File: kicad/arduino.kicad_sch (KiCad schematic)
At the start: 23 parts, among them J1 USB_B, J2 Conn_02x03_Odd_Even, SW1 Reset, U5 ATmega328P-A, U6 CH340C, U7 AMS1117-5.0, Y1 16MHz

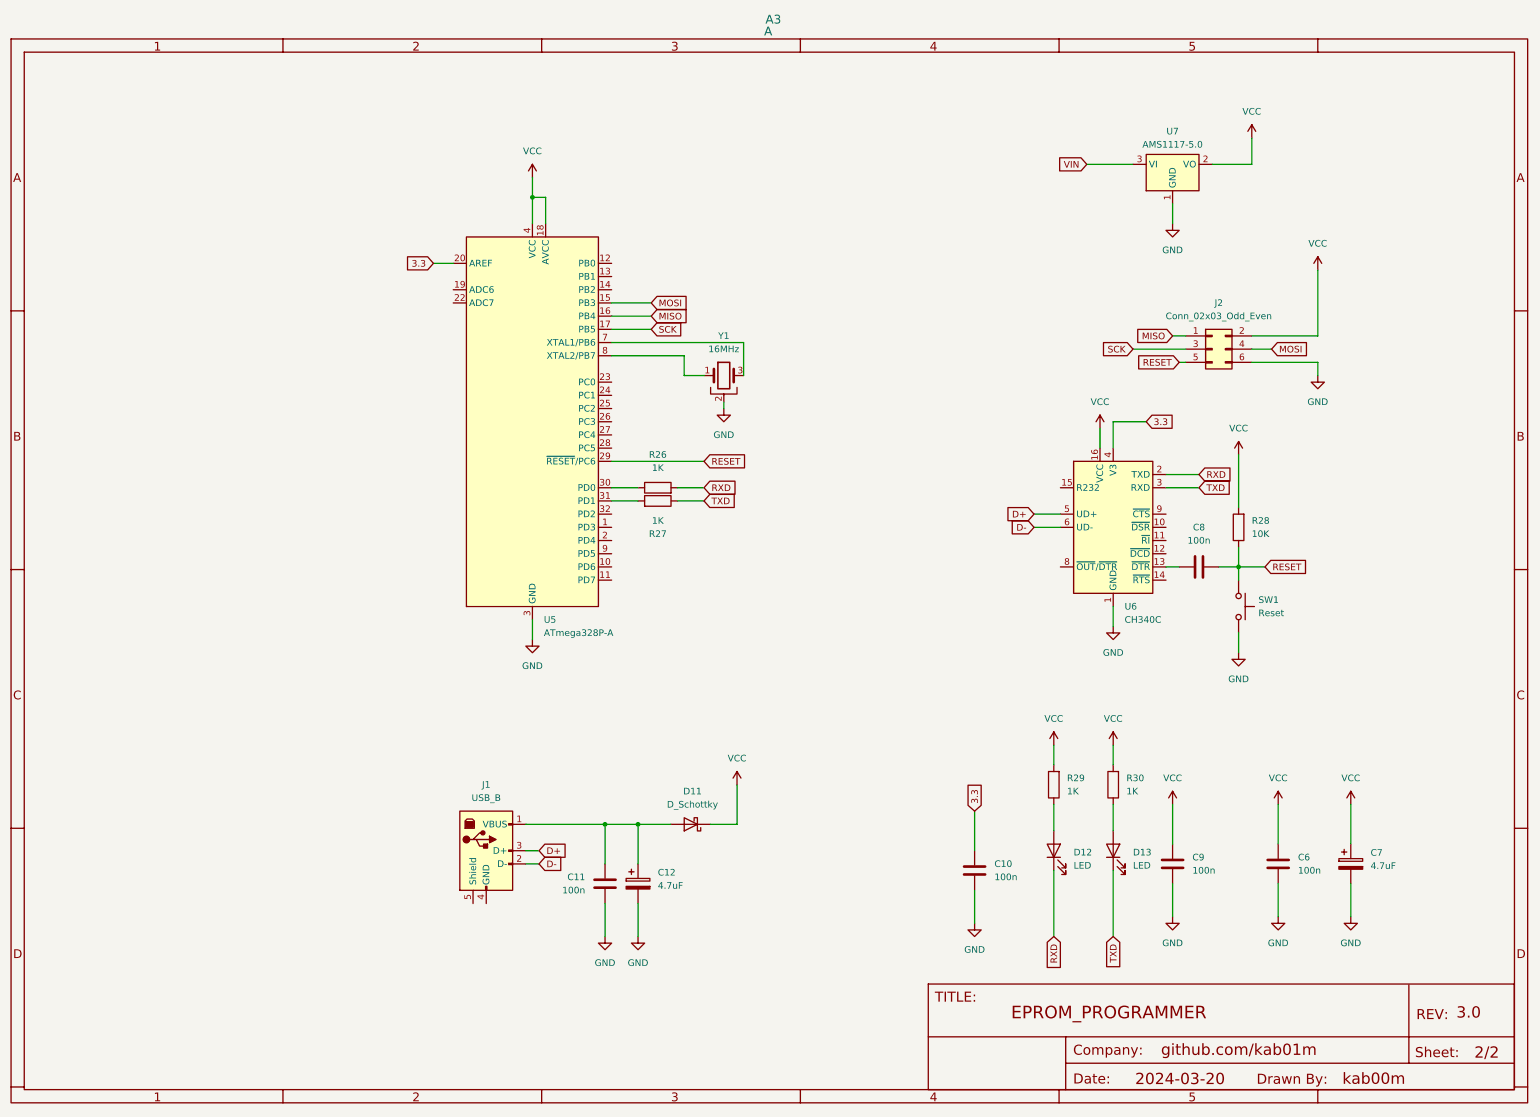
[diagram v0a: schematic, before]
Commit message: Small pre-release fixes
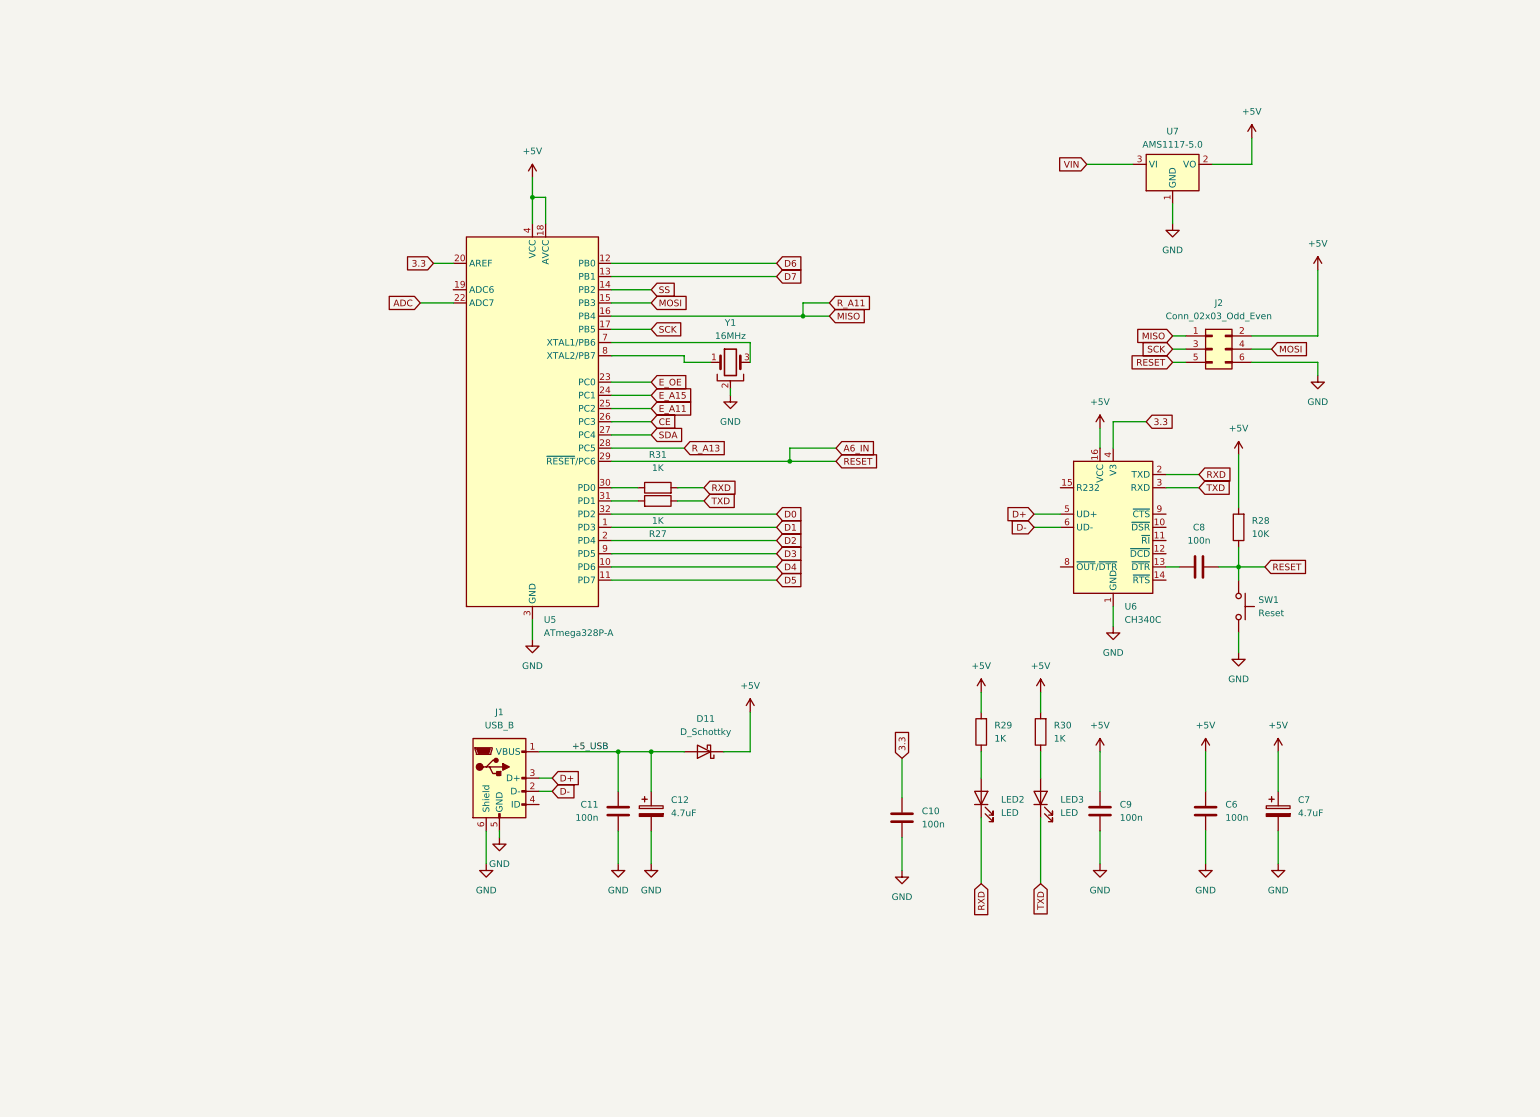
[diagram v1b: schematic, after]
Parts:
- removed A3: A, symbol Unknown_20_-821
- C12, C7: footprint Capacitor_Tantalum_SMD:CP_EIA-7361-38_AVX-V_Pad2.18x3.30mm_HandSolder -> Capacitor_Tantalum_SMD:CP_EIA-3216-18_Kemet-A_Pad1.58x1.35mm_HandSolder
- J1: symbol Connector:USB_B -> Connector:USB_B_Micro
- J2: footprint Connector_IDC:IDC-Header_2x03_P2.54mm_Vertical -> Connector_PinHeader_2.54mm:PinHeader_2x03_P2.54mm_Vertical
- SW1: footprint Button_Switch_SMD:Nidec_Copal_SH-7010A -> Button_Switch_SMD:SW_SPST_TL3342
- Y1: footprint Crystal:Resonator_SMD_Murata_CSTxExxV-3Pin_3.0x1.1mm_HandSoldering -> Crystal:Resonator_SMD_Murata_CSTxExxV-3Pin_3.0x1.1mm
- renumbered D12 to LED2, D13 to LED3, R26 to R31
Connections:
- net GND: now also J1.5 (GND), J1.6 (Shield)
- net +5_USB: now reaches C11.1, C12.1, D11.2 (A), J1.1 (VBUS)
- net D1: now reaches U5.1 (PD3)
- net D4: now reaches U5.10 (PD6)
- net D5: now reaches U5.11 (PD7)
- net D6: now reaches U5.12 (PB0)
- net D7: now reaches U5.13 (PB1)
- net SS: now reaches U5.14 (PB2)
- net D2: now reaches U5.2 (PD4)
- net ADC: now reaches U5.22 (ADC7)
- net E_OE: now reaches U5.23 (PC0)
- net E_A15: now reaches U5.24 (PC1)
- net E_A11: now reaches U5.25 (PC2)
- net CE: now reaches U5.26 (PC3)
- net SDA: now reaches U5.27 (PC4)
- net R_A13: now reaches U5.28 (PC5)
- net D0: now reaches U5.32 (PD2)
- net D3: now reaches U5.9 (PD5)
- net RESET renamed A6_IN
- net VCC renamed +5V
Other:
- company: (none) -> kab01m@github
- title: (none) -> EPROM27 Arduino programmer
- moved on the sheet: C10, C11, C12, C6, C7, C9, D11, LED2, LED3, R29, R30, Y1
